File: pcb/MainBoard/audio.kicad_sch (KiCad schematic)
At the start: 6 parts

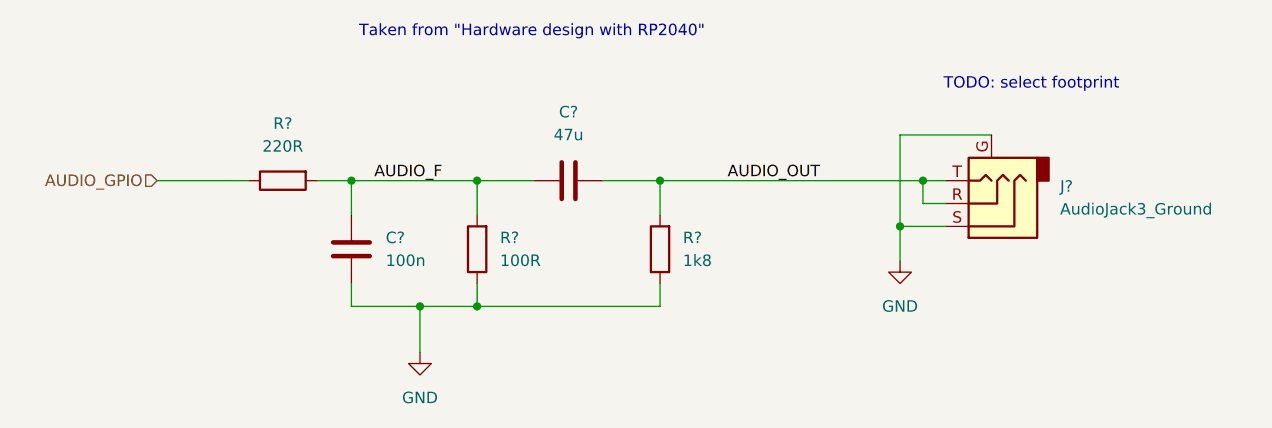
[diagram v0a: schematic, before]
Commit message: pcb: main board - contd
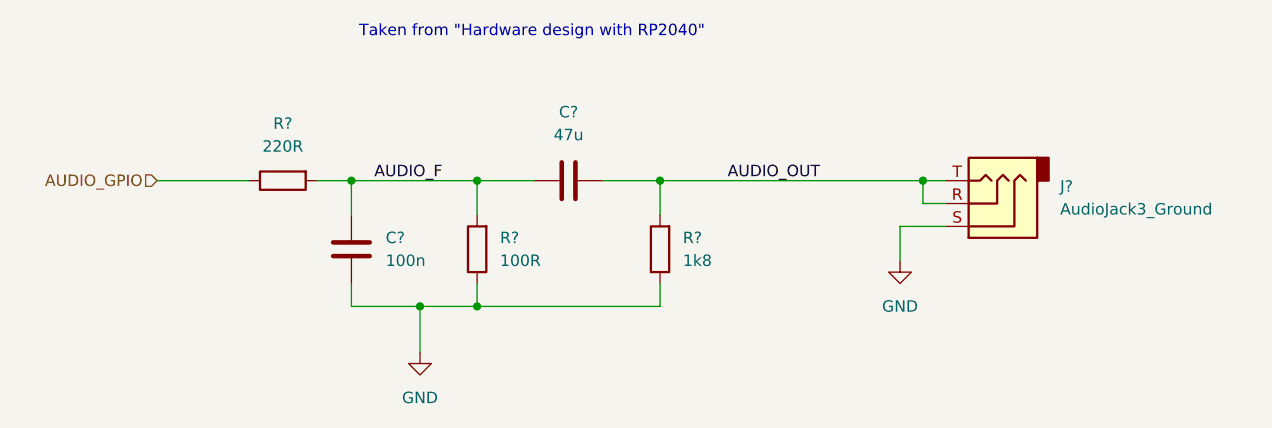
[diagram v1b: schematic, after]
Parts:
- J?: footprint (none) -> led-matrix:3.5mm-audio-jack; symbol Connector_Audio:AudioJack3_Ground -> Connector_Audio:AudioJack3
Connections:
- net GND: no longer J?.G
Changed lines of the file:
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@@
-	)
-	(junction
-		(at 130.81 52.07)
-		(diameter 0)
-		(color 0 0 0 0)
 	)
 	(junction
@@
 	(wire
 		(pts
-			(xy 130.81 41.91) (xy 130.81 52.07)
-		)
-		(stroke
-			(width 0)
-			(type default)
-		)
-	)
-	(wire
-		(pts
 			(xy 83.82 60.96) (xy 104.14 60.96)
 		)
@@
 	(wire
 		(pts
-			(xy 140.97 41.91) (xy 130.81 41.91)
-		)
-		(stroke
-			(width 0)
-			(type default)
-		)
-	)
-	(wire
-		(pts
 			(xy 133.35 46.99) (xy 135.89 46.99)
 		)
@@
 			(width 0)
 			(type default)
-		)
-	)
-	(text_box "TODO: select footprint"
-		(exclude_from_sim no)
-		(at 134.62 34.29 0)
-		(size 30.48 3.81)
-		(stroke
-			(width -0.0001)
-			(type default)
-		)
-		(fill
-			(type none)
-		)
-		(effects
-			(font
-				(size 1.27 1.27)
-			)
-			(justify left top)
 		)
 	)
@@
 	)
 	(symbol
-		(lib_id "Connector_Audio:AudioJack3_Ground")
+		(lib_id "Connector_Audio:AudioJack3")
 		(at 140.97 49.53 180)
 		(unit 1)
@@
 			)
 		)
-		(property "Footprint" ""
+		(property "Footprint" "led-matrix:3.5mm-audio-jack"
 			(at 140.97 49.53 0)
 			(effects
@@
 			)
 		)
-		(property "Description" "Audio Jack, 3 Poles (Stereo / TRS), Grounded Sleeve"
+		(property "Description" "Audio Jack, 3 Poles (Stereo / TRS)"
 			(at 140.97 49.53 0)
 			(effects
@@
 		(pin "R"
 		)
-		(pin "G"
-		)
 		(pin "S"
